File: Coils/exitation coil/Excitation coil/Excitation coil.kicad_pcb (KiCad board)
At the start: 2 copper layers, 74.8 x 56.5 mm, 6 parts, among them J1 Conn_01x04

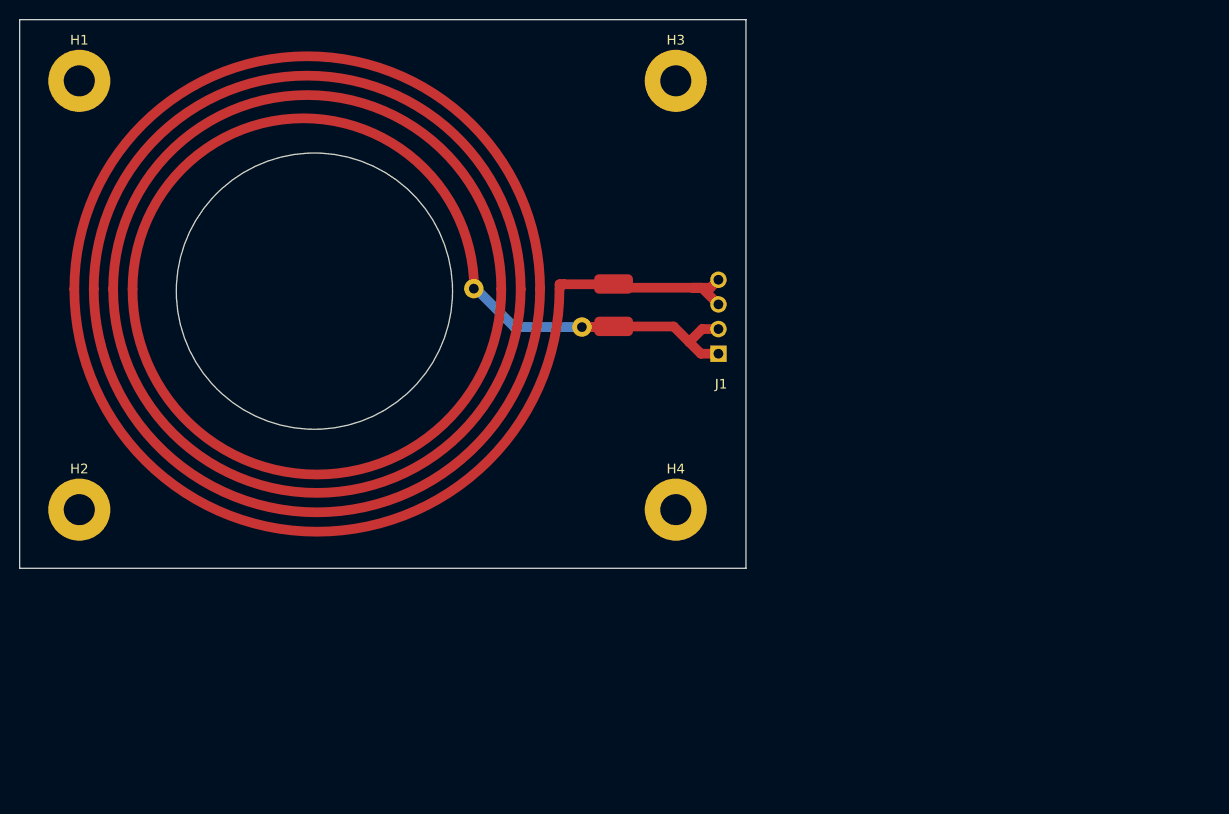
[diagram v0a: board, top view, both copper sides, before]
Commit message: Final version before review 3
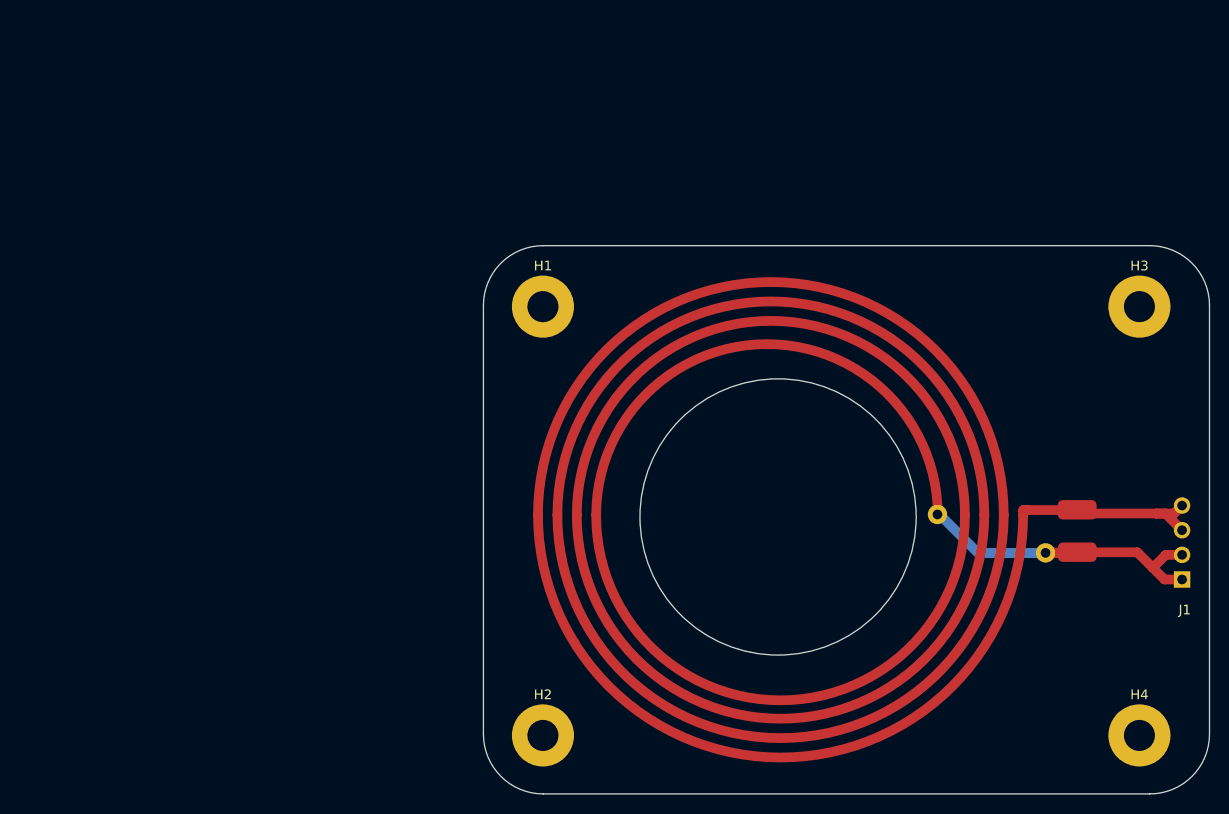
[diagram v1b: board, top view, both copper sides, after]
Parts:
- moved H2 53.1 mm to (156.1, 150.5)
- moved H1 53.1 mm to (156.1, 106.3)
- moved H3 53.1 mm to (217.6, 106.3)
- moved H4 53.1 mm to (217.6, 150.5)
- moved REF** 53.1 mm to (179.6, 127.8)
- moved J1 53.1 mm to (222.0, 134.4)
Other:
- outline, holes or cut-outs redrawn
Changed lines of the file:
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@@
 	(footprint "MountingHole:MountingHole_3.2mm_M3_Pad"
 		(layer "F.Cu")
-		(at 169.8359 83.035)
+		(at 217.6168 106.3052)
 		(descr "Mounting Hole 3.2mm, M3")
 		(tags "mounting hole 3.2mm m3")
@@
 	(footprint "MountingHole:MountingHole_3.2mm_M3_Pad"
 		(layer "F.Cu")
-		(at 169.8359 127.225)
+		(at 217.6168 150.4952)
 		(descr "Mounting Hole 3.2mm, M3")
 		(tags "mounting hole 3.2mm m3")
@@
 	(footprint "MountingHole:MountingHole_3.2mm_M3_Pad"
 		(layer "F.Cu")
-		(at 108.3659 127.225)
+		(at 156.1468 150.4952)
 		(descr "Mounting Hole 3.2mm, M3")
 		(tags "mounting hole 3.2mm m3")
@@
 	(footprint "Top sensing coik"
 		(layer "F.Cu")
-		(at 131.8534 104.5)
+		(at 179.6343 127.7702)
 		(property "Reference" "REF**"
 			(at 0 0 0)
@@
 	(footprint "MountingHole:MountingHole_3.2mm_M3_Pad"
 		(layer "F.Cu")
-		(at 108.3659 83.035)
+		(at 156.1468 106.3052)
 		(descr "Mounting Hole 3.2mm, M3")
 		(tags "mounting hole 3.2mm m3")
@@
 	(footprint "Connector_PinHeader_2.54mm:PinHeader_1x04_P2.54mm_Horizontal"
 		(layer "B.Cu")
-		(at 174.2309 111.155)
+		(at 222.0118 134.4252)
 		(descr "Through hole angled pin header, 1x04, 2.54mm pitch, 6mm pin length, single row")
 		(tags "Through hole angled pin header THT 1x04 2.54mm single row")
@@
 		)
 	)
-	(gr_rect
-		(start 102.2191 76.7298)
-		(end 177.0691 133.2702)
+	(gr_arc
+		(start 156.173075 156.520727)
+		(mid 151.816925 154.71635)
+		(end 150.012548 150.3602)
 		(stroke
 			(width 0.05)
 			(type default)
 		)
-		(fill none)
 		(layer "Edge.Cuts")
 	)
-	(gr_circle
-		(center 132.5975 104.708697)
-		(end 144.9759 97.685)
+	(gr_line
+		(start 150.012548 150.3602)
+		(end 150.012548 106.1802)
 		(stroke
 			(width 0.05)
 			(type default)
 		)
+		(layer "Edge.Cuts")
+	)
+	(gr_arc
+		(start 150.012548 106.1802)
+		(mid 151.816925 101.82405)
+		(end 156.173075 100.019673)
+		(stroke
+			(width 0.05)
+			(type default)
+		)
+		(layer "Edge.Cuts")
+	)
+	(gr_arc
+		(start 218.676925 100.019673)
+		(mid 223.033075 101.82405)
+		(end 224.837452 106.1802)
+		(stroke
+			(width 0.05)
+			(type default)
+		)
+		(layer "Edge.Cuts")
+	)
+	(gr_line
+		(start 224.837452 106.1802)
+		(end 224.837452 150.3602)
+		(stroke
+			(width 0.05)
+			(type default)
+		)
+		(layer "Edge.Cuts")
+	)
+	(gr_arc
+		(start 224.837452 150.3602)
+		(mid 223.033075 154.71635)
+		(end 218.676925 156.520727)
+		(stroke
+			(width 0.05)
+			(type default)
+		)
+		(layer "Edge.Cuts")
+	)
+	(gr_circle
+		(center 180.3784 127.978897)
+		(end 192.7568 120.9552)
+		(stroke
+			(width 0.05)
+			(type default)
+		)
 		(fill none)
+		(layer "Edge.Cuts")
+	)
+	(gr_line
+		(start 156.173075 156.520727)
+		(end 218.676925 156.520727)
+		(stroke
+			(width 0.05)
+			(type default)
+		)
+		(layer "Edge.Cuts")
+	)
+	(gr_line
+		(start 156.173075 100.019673)
+		(end 218.676925 100.019673)
+		(stroke
+			(width 0.05)
+			(type default)
+		)
 		(layer "Edge.Cuts")
 	)
@@
 		(layer "User.1")
 		(pts
-			(xy 102.2191 133.2702) (xy 102.2191 76.7298)
+			(xy 150 156.5404) (xy 150 100)
 		)
 		(height -34.5091)
 		(gr_text "56.5404 mm"
-			(at 66.56 105 90)
+			(at 114.3409 128.2702 90)
 			(layer "User.1")
 			(effects
@@
 		(layer "User.1")
 		(pts
-			(xy 102.2191 76.7298) (xy 177.0691 76.7298)
+			(xy 150 100) (xy 224.85 100)
 		)
 		(height -31.2798)
 		(gr_text "74.8500 mm"
-			(at 139.6441 44.3 0)
+			(at 187.425 67.5702 0)
 			(layer "User.1")
 			(effects
@@
 	)
 	(segment
-		(start 172.5109 104.355)
-		(end 171.5659 104.355)
+		(start 220.2918 127.6252)
+		(end 219.3468 127.6252)
 		(width 1)
 		(layer "F.Cu")
@@
 	)
 	(segment
-		(start 163.4234 103.97)
-		(end 163.8084 104.355)
+		(start 211.2043 127.2402)
+		(end 211.5893 127.6252)
 		(width 1)
 		(layer "F.Cu")
@@
 	)
 	(segment
-		(start 173.4109 104.355)
-		(end 174.2309 103.535)
+		(start 221.1918 127.6252)
+		(end 222.0118 126.8052)
 		(width 1)
 		(layer "F.Cu")
@@
 	)
 	(segment
-		(start 171.5659 104.355)
-		(end 173.4109 104.355)
+		(start 219.3468 127.6252)
+		(end 221.1918 127.6252)
 		(width 1)
 		(layer "F.Cu")
@@
 	)
 	(segment
-		(start 163.8084 104.355)
-		(end 171.5659 104.355)
+		(start 211.5893 127.6252)
+		(end 219.3468 127.6252)
 		(width 1)
 		(layer "F.Cu")
@@
 	)
 	(segment
-		(start 174.2309 106.075)
-		(end 172.5109 104.355)
+		(start 222.0118 129.3452)
+		(end 220.2918 127.6252)
 		(width 1)
 		(layer "F.Cu")
@@
 	)
 	(segment
-		(start 171.2159 109.95)
-		(end 172.4209 111.155)
+		(start 218.9968 133.2202)
+		(end 220.2018 134.4252)
 		(width 1)
 		(layer "F.Cu")
@@
 	)
 	(segment
-		(start 172.5509 108.615)
-		(end 174.2309 108.615)
+		(start 220.3318 131.8852)
+		(end 222.0118 131.8852)
 		(width 1)
 		(layer "F.Cu")
@@
 	)
 	(segment
-		(start 169.6159 108.35)
-		(end 171.2159 109.95)
+		(start 217.3968 131.6202)
+		(end 218.9968 133.2202)
 		(width 1)
 		(layer "F.Cu")
@@
 	)
 	(segment
-		(start 163.4334 108.34)
-		(end 163.4434 108.35)
+		(start 211.2143 131.6102)
+		(end 211.2243 131.6202)
 		(width 1)
 		(layer "F.Cu")
@@
 	)
 	(segment
-		(start 171.2159 109.95)
-		(end 172.5509 108.615)
+		(start 218.9968 133.2202)
+		(end 220.3318 131.8852)
 		(width 1)
 		(layer "F.Cu")
@@
 	)
 	(segment
-		(start 163.4434 108.35)
-		(end 169.6159 108.35)
+		(start 211.2243 131.6202)
+		(end 217.3968 131.6202)
 		(width 1)
 		(layer "F.Cu")
@@
 	)
 	(segment
-		(start 172.4209 111.155)
-		(end 174.2309 111.155)
+		(start 220.2018 134.4252)
+		(end 222.0118 134.4252)
 		(width 1)
 		(layer "F.Cu")
@@
 	)
 	(group ""
-		(members "0983a8b6-e05b-4e90-86f0-2ec26d8243b9" "1b1254fa-3e5b-426d-af85-557729cb2266"
-			"1dc95f1f-9eb9-46d5-92c7-d03396abb6e8" "2a3e1d69-24b1-4367-96ef-8026e52f77d9"
-			"34ce22b7-6f16-4384-83a5-7ea790f4913c" "3b179f83-0c2d-48d1-92e6-6b90469de76e"
-			"40f66516-42ef-430a-a015-479538c62a99" "620ee7d5-88e1-42c2-8c6c-2b91265c4c2c"
+		(members "0983a8b6-e05b-4e90-86f0-2ec26d8243b9" "1aff5de9-3b05-48e9-9b56-f04d94e861d0"
+			"1b1254fa-3e5b-426d-af85-557729cb2266" "1dc95f1f-9eb9-46d5-92c7-d03396abb6e8"
+			"2a3e1d69-24b1-4367-96ef-8026e52f77d9" "34ce22b7-6f16-4384-83a5-7ea790f4913c"
+			"3b179f83-0c2d-48d1-92e6-6b90469de76e" "40f66516-42ef-430a-a015-479538c62a99"
 			"67f27e21-539c-4e19-b3d7-59ecd18bddae" "78d8a6bc-3c50-44d7-93f9-978656f11ed5"
 			"7af8a61a-6e76-4a78-ba0c-0efa05c25db2" "824b128f-ff58-4802-b877-6a3ad7580c26"
@@
 		)
 	)
+	(group ""
+		(members "023d86c4-9d62-4667-b599-cfe0c7d6919f" "31665cbc-dee6-4b45-81da-e014d1a65e6d"
+			"3c2b62f7-c912-4d64-92ca-1ecbb0c29d48" "40d2eea9-5a91-4822-8024-619dfa8afd4d"
+			"6da2f96f-3e4a-4d81-b892-a9bc27639868" "9966aed0-e3de-4a79-a706-083d00f72100"
+			"e6c3b0f1-3c05-4d5f-88c0-1e10e4b1e0e9" "fb88849c-2a93-45af-b330-d60495a1f3bb"
+		)
+	)
